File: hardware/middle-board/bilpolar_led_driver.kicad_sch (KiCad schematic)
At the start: 2 parts, among them U2 TL074

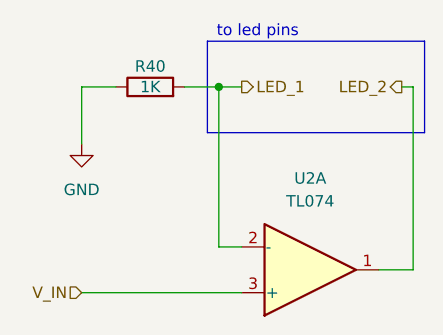
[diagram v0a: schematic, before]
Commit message: wip - first pass done
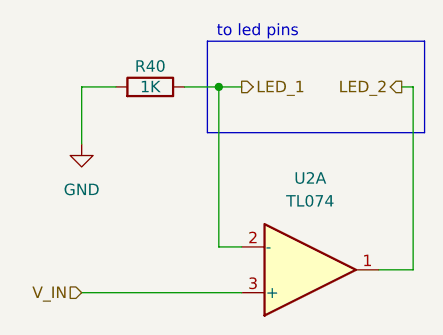
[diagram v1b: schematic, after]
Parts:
- R40: footprint Resistor_THT:R_Axial_DIN0207_L6.3mm_D2.5mm_P7.62mm_Horizontal -> Eurorack Common:R_Axial_DIN0207_L6.3mm_D2.5mm_P7.62mm_Horizontal; symbol Device:R -> Eurorack Common:R_DIN0207
- U2: footprint Package_DIP:DIP-14_W7.62mm -> Eurorack Common:DIP-14_W7.62mm; symbol Amplifier_Operational:TL074 -> Eurorack Common:TL074CN
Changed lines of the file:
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@@
 	)
 	(symbol
-		(lib_id "Amplifier_Operational:TL074")
+		(lib_id "Eurorack Common:TL074CN")
 		(at 78.74 87.63 0)
 		(mirror x)
@@
 			)
 		)
-		(property "Footprint" "Package_DIP:DIP-14_W7.62mm"
+		(property "Footprint" "Eurorack Common:DIP-14_W7.62mm"
 			(at 77.47 90.17 0)
 			(effects
@@
 			)
 		)
-		(property "Datasheet" "http://www.ti.com/lit/ds/symlink/tl071.pdf"
+		(property "Datasheet" "http://www.ti.com/lit/ds/symlink/tl074.pdf"
 			(at 80.01 92.71 0)
 			(effects
@@
 			)
 		)
-		(property "Description" "Quad Low-Noise JFET-Input Operational Amplifiers, DIP-14/SOIC-14"
+		(property "Description" "Quad Low-Noise JFET-Input Operational Amplifiers, DIP-14"
 			(at 78.74 87.63 0)
 			(effects
@@
 	)
 	(symbol
-		(lib_id "Device:R")
+		(lib_id "Eurorack Common:R_DIN0207")
 		(at 60.96 67.31 90)
 		(unit 1)
@@
 			)
 		)
-		(property "Footprint" "Resistor_THT:R_Axial_DIN0207_L6.3mm_D2.5mm_P7.62mm_Horizontal"
+		(property "Footprint" "Eurorack Common:R_Axial_DIN0207_L6.3mm_D2.5mm_P7.62mm_Horizontal"
 			(at 60.96 69.088 90)
 			(effects
